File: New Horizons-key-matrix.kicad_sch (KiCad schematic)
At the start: 144 parts, among them J1 Conn_01x09_Socket, J2 Conn_01x09_Socket, J3 Conn_01x05_Socket, SW1 SW_Push, SW10 SW_Push, SW11 SW_Push, SW12 SW_Push, SW13 SW_Push, SW14 SW_Push, SW15 SW_Push, SW16 SW_Push, SW17 SW_Push, SW18 SW_Push, SW19 SW_Push, SW2 SW_Push, SW20 SW_Push, SW21 SW_Push, SW22 SW_Push, SW23 SW_Push, SW24 SW_Push, SW25 SW_Push, SW26 SW_Push, SW27 SW_Push, SW28 SW_Push, SW29 SW_Push, SW3 SW_Push, SW30 SW_Push, SW31 SW_Push, SW32 SW_Push, SW33 SW_Push, SW34 SW_Push, SW35 SW_Push, SW36 SW_Push, SW37 SW_Push, SW38 SW_Push, SW39 SW_Push, SW4 SW_Push, SW40 SW_Push, SW41 SW_Push, SW42 SW_Push, SW43 SW_Push, SW44 SW_Push, SW45 SW_Push, SW46 SW_Push, SW47 SW_Push, SW48 SW_Push, SW49 SW_Push, SW5 SW_Push, SW50 SW_Push, SW51 SW_Push, SW52 SW_Push, SW53 SW_Push, SW54 SW_Push, SW55 SW_Push, SW56 SW_Push, SW57 SW_Push, SW58 SW_Push, SW59 SW_Push, SW6 SW_Push, SW60 SW_Push, SW61 SW_Push, SW62 SW_Push, SW63 SW_Push, SW64 SW_Push, SW65 SW_Push, SW66 SW_Push, SW67 SW_Push, SW68 SW_Push, SW7 SW_Push, SW8 SW_Push, SW9 SW_Push

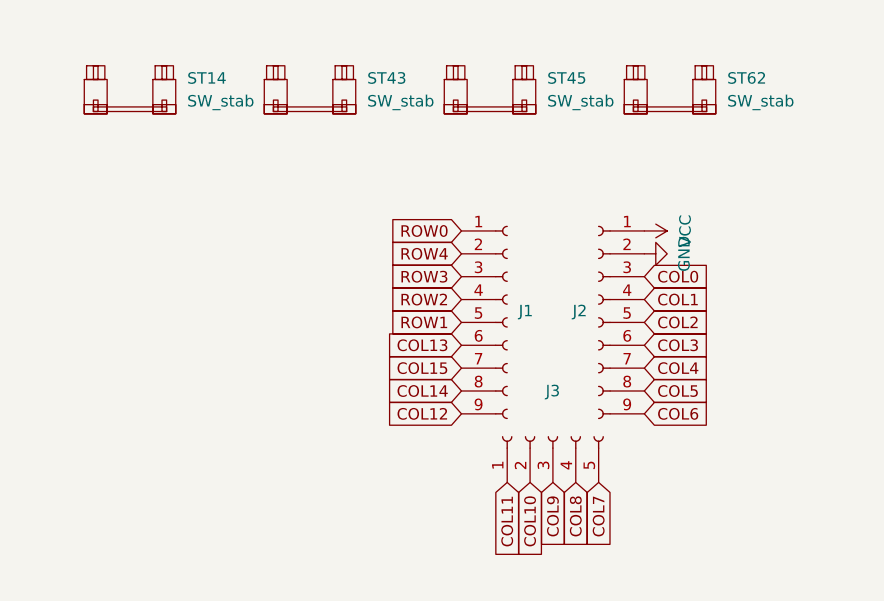
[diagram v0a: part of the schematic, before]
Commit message: work
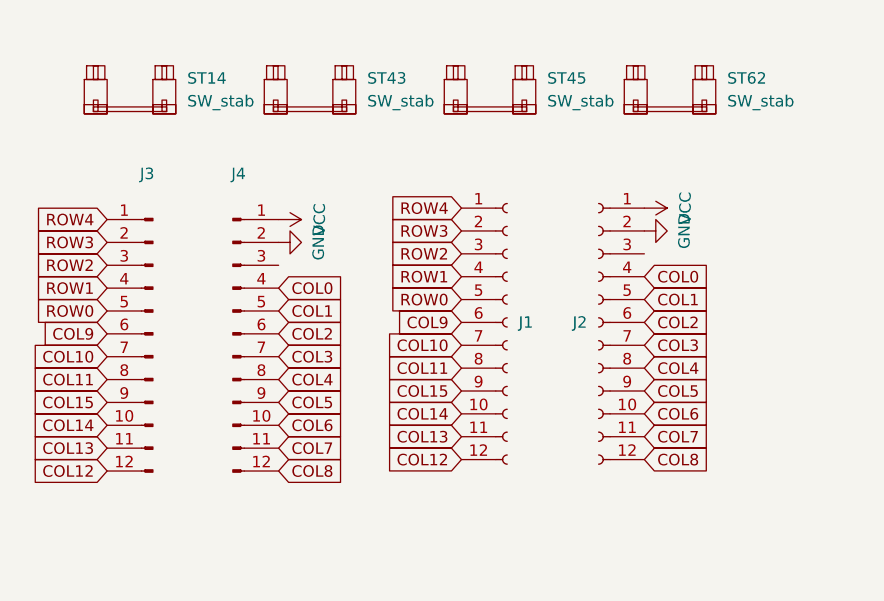
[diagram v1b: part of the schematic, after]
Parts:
- removed J1, J2: Conn_01x09_Socket, Connector_PinHeader_2.54mm:PinHeader_1x09_P2.54mm_Vertical, symbol Connector:Conn_01x09_Socket
- removed J3: Conn_01x05_Socket, Connector_PinHeader_2.54mm:PinHeader_1x05_P2.54mm_Vertical, symbol Connector:Conn_01x05_Socket
- added J1, J2: Conn_01x12_Socket, Connector_PinSocket_2.54mm:PinSocket_1x12_P2.54mm_Vertical, symbol Connector:Conn_01x12_Socket
- added J3, J4: Conn_01x12_Pin, Connector_PinHeader_2.54mm:PinHeader_1x12_P2.54mm_Vertical, symbol Connector:Conn_01x12_Pin
- Gemini1: value ~ -> (none)
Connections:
- net COL0: now also J2.4 (Pin_4), J4.4 (Pin_4)
- net COL1: now also J2.5 (Pin_5), J4.5 (Pin_5)
- net COL10: now also J1.7 (Pin_7), J3.7 (Pin_7)
- net COL11: now also J1.8 (Pin_8), J3.8 (Pin_8)
- net COL12: now also J1.12 (Pin_12), J3.12 (Pin_12)
- net COL13: now also J1.11 (Pin_11), J3.11 (Pin_11)
- net COL14: now also J1.10 (Pin_10), J3.10 (Pin_10)
- net COL15: now also J1.9 (Pin_9), J3.9 (Pin_9)
- net COL2: now also J2.6 (Pin_6), J4.6 (Pin_6)
- net COL3: now also J2.7 (Pin_7), J4.7 (Pin_7)
- net COL4: now also J2.8 (Pin_8), J4.8 (Pin_8)
- net COL5: now also J2.9 (Pin_9), J4.9 (Pin_9)
- net COL6: now also J2.10 (Pin_10), J4.10 (Pin_10)
- net COL7: now also J2.11 (Pin_11), J4.11 (Pin_11)
- net COL8: now also J2.12 (Pin_12), J4.12 (Pin_12)
- net COL9: now also J1.6 (Pin_6), J3.6 (Pin_6)
- net GND: now also J2.2 (Pin_2), J4.2 (Pin_2)
- net ROW0: now also J1.5 (Pin_5), J3.5 (Pin_5)
- net ROW1: now also J1.4 (Pin_4), J3.4 (Pin_4)
- net ROW2: now also J1.3 (Pin_3), J3.3 (Pin_3)
- net ROW3: now also J1.2 (Pin_2), J3.2 (Pin_2)
- net ROW4: now also J1.1 (Pin_1), J3.1 (Pin_1)
- net VCC: now also J2.1 (Pin_1), J4.1 (Pin_1)

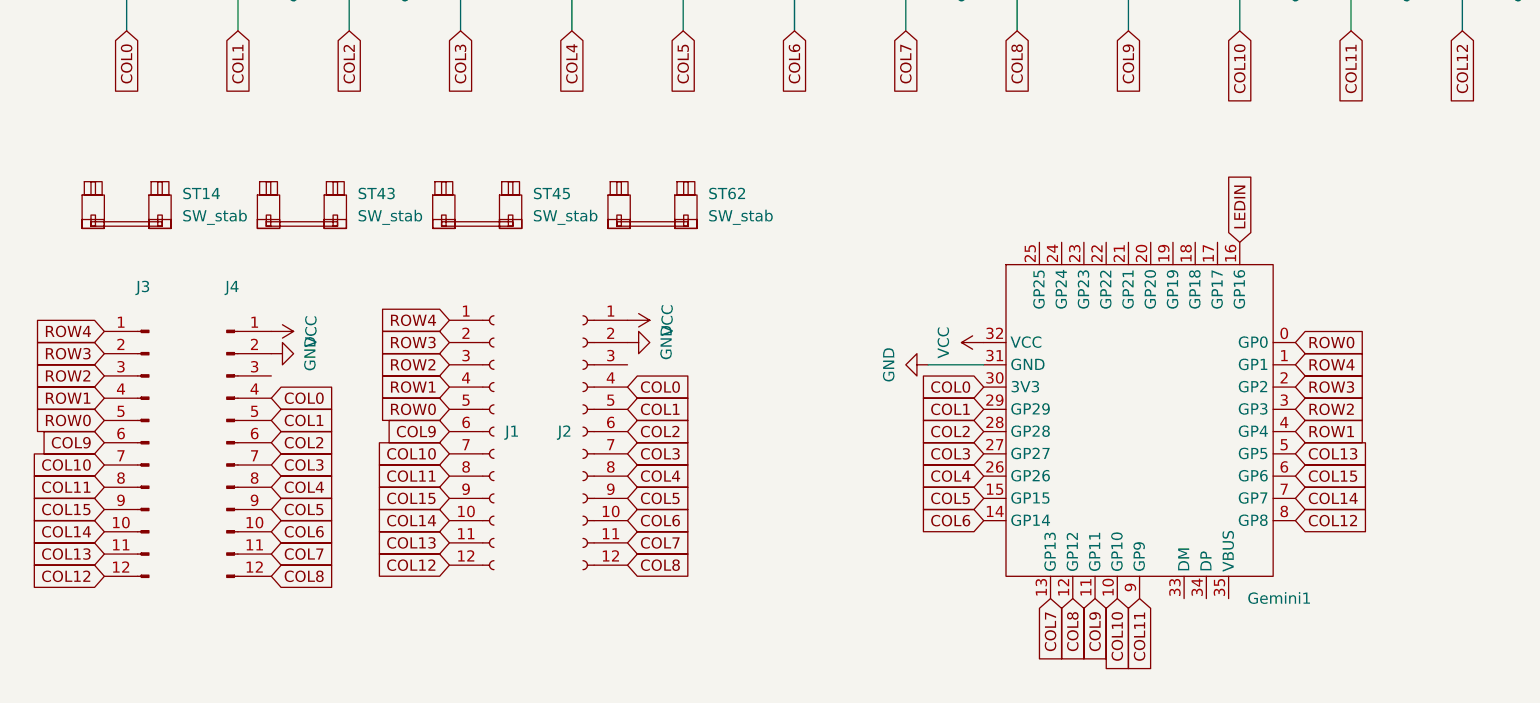
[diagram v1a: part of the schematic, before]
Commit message: progress
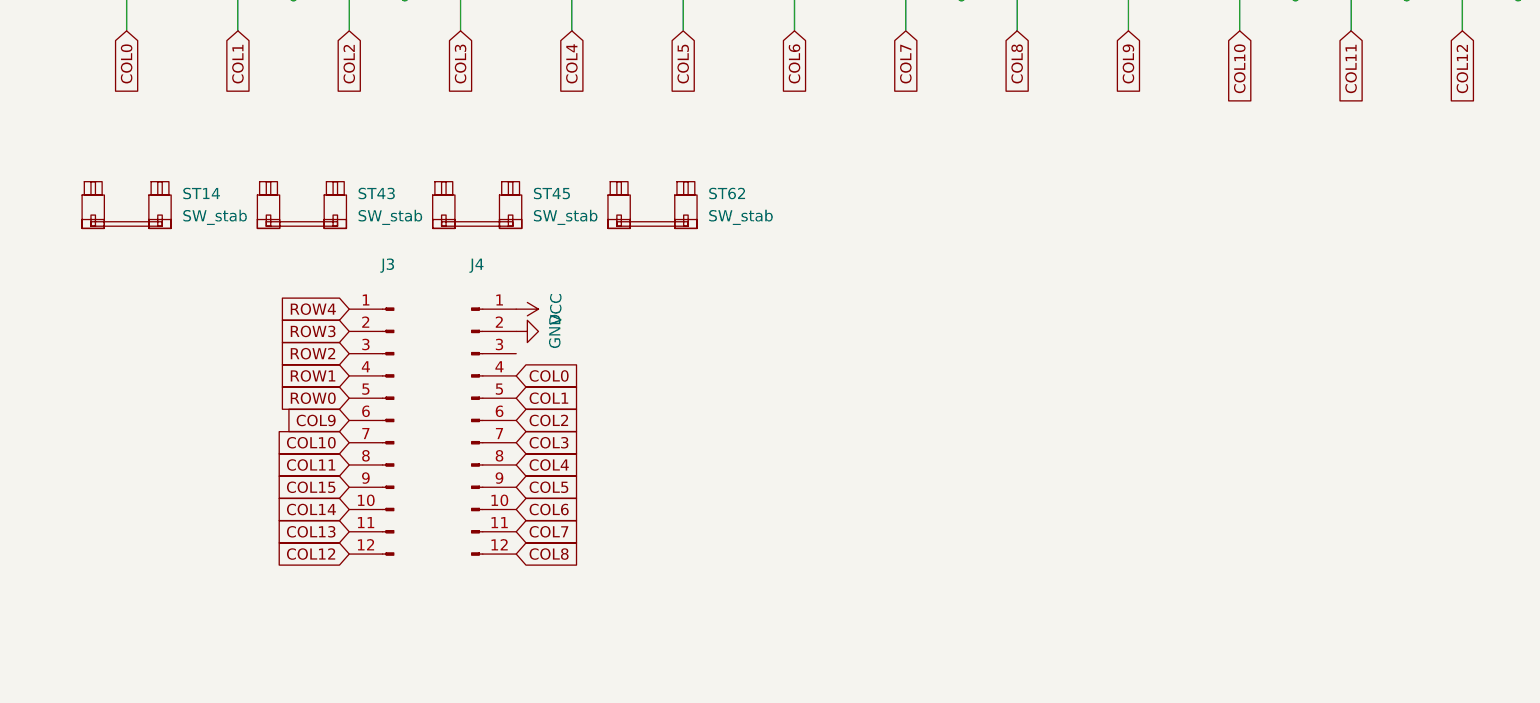
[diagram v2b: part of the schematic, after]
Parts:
- removed Gemini1: (no value), Gemini:gemini, symbol local:gemini
- removed J1, J2: Conn_01x12_Socket, Connector_PinSocket_2.54mm:PinSocket_1x12_P2.54mm_Vertical, symbol Connector:Conn_01x12_Socket
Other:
- moved on the sheet: J3, J4
